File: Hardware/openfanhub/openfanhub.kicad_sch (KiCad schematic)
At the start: 60 parts, among them J1 UART, J2 I2C, J3 12V in, J4 GND in, J5 5V IN, J6 SWD, U1 STM32F103C8T8_Board, U2 STM32F103C8Tx, U3 AMS1117, U4 USBLC6-2SC6, U5 AMS1117, U6 USB_HEADER_IN, U7 USB_HEADER_OUT, Y1 Crystal

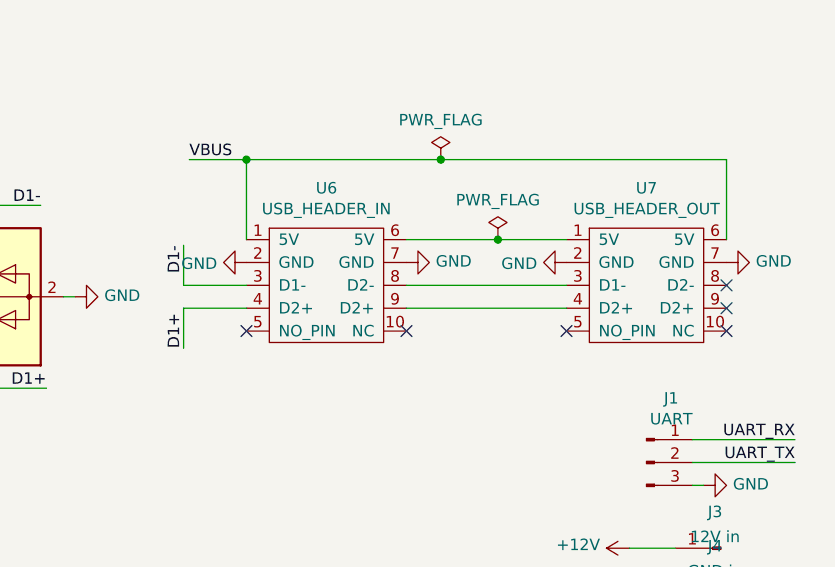
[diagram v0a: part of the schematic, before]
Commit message: update
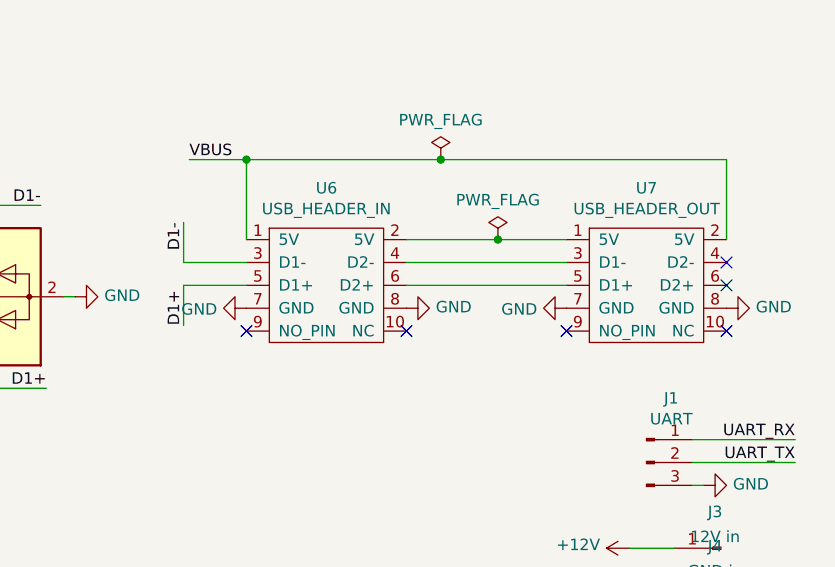
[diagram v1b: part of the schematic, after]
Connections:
- net D1+: now also U6.5 (D1+); no longer U6.4 (D2+)
- net GND: now also U6.8 (GND), U7.8 (GND); no longer U6.2 (GND), U7.2 (GND)
- net VBUS: now also U7.2 (5V); no longer U7.6 (5V)
- net at U7.1 (5V): now also U6.2 (5V); no longer U6.6 (5V)
- net at U7.3 (D1-): now also U6.4 (D2-); no longer U6.8 (D2-)
- net at U6.9 (NO_PIN): no longer U7.4 (D2+)
- net at U7.5 (D1+): now also U6.6 (D2+)
